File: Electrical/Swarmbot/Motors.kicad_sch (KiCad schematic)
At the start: 8 parts, among them J6 Motor 1, J7 Motor 2, U10 MPC17531A

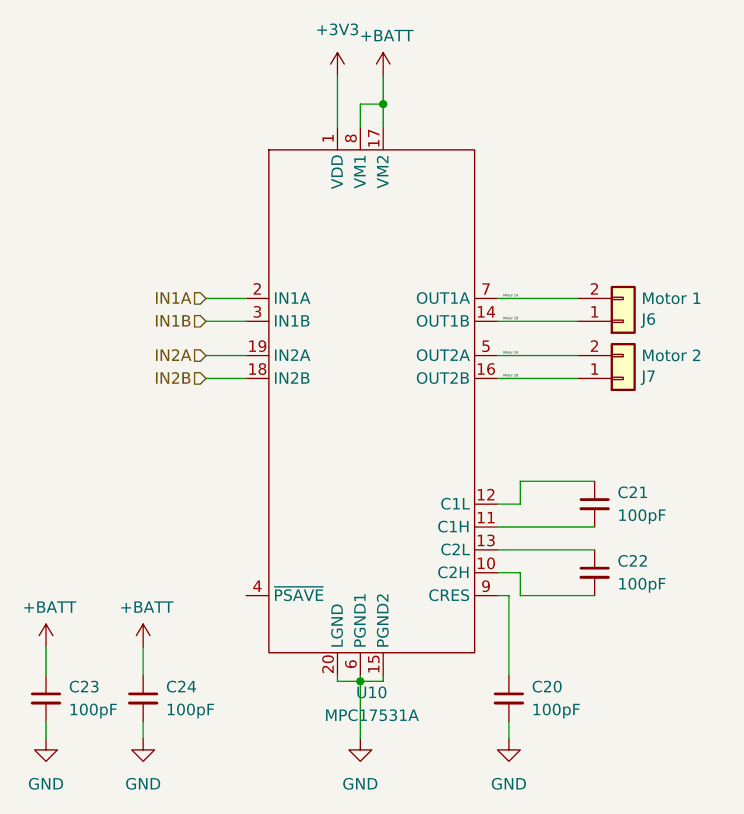
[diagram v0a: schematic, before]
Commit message: some little changes have been made
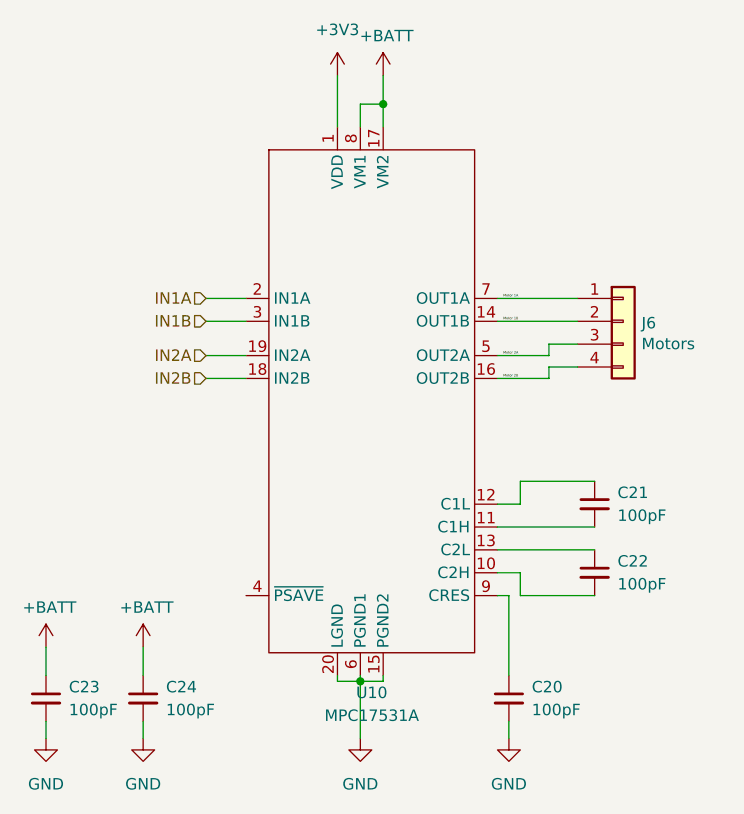
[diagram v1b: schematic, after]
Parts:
- removed J6: Motor 1, Connector_JST:JST_XH_B2B-XH-AM_1x02_P2.50mm_Vertical, symbol Connector_Generic:Conn_01x02
- removed J7: Motor 2, Connector_JST:JST_XH_B2B-XH-AM_1x02_P2.50mm_Vertical, symbol Connector_Generic:Conn_01x02
- added J6: Motors, Connector_JST:JST_XH_B4B-XH-AM_1x04_P2.50mm_Vertical, symbol Connector_Generic:Conn_01x04
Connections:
- net Motor 1A: now also J6.1 (Pin_1)
- net Motor 1B: now also J6.2 (Pin_2)
- net Motor 2A: now also J6.3 (Pin_3)
- net Motor 2B: now also J6.4 (Pin_4)
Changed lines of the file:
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@@
     (stroke (width 0) (type default) (color 0 0 0 0))
   )
-  (wire (pts (xy 126.365 83.185) (xy 135.255 83.185))
-    (stroke (width 0) (type default) (color 0 0 0 0))
-  )
-  (wire (pts (xy 126.365 85.725) (xy 135.255 85.725))
+  (wire (pts (xy 126.365 83.185) (xy 132.08 83.185))
+    (stroke (width 0) (type default) (color 0 0 0 0))
+  )
+  (wire (pts (xy 126.365 85.725) (xy 132.08 85.725))
     (stroke (width 0) (type default) (color 0 0 0 0))
   )
@@
   )
   (wire (pts (xy 128.905 109.855) (xy 137.16 109.855))
+    (stroke (width 0) (type default) (color 0 0 0 0))
+  )
+  (wire (pts (xy 132.08 81.915) (xy 132.08 83.185))
+    (stroke (width 0) (type default) (color 0 0 0 0))
+  )
+  (wire (pts (xy 132.08 84.455) (xy 132.08 85.725))
+    (stroke (width 0) (type default) (color 0 0 0 0))
+  )
+  (wire (pts (xy 135.255 81.915) (xy 132.08 81.915))
+    (stroke (width 0) (type default) (color 0 0 0 0))
+  )
+  (wire (pts (xy 135.255 84.455) (xy 132.08 84.455))
     (stroke (width 0) (type default) (color 0 0 0 0))
   )
@@
     (pin "2")
   )
-  (symbol (lib_id "Connector_Generic:Conn_01x02") (at 140.335 79.375 0) (mirror x) (unit 1)
-    (in_bom yes) (on_board yes)
-    (property "Reference" "J6" (id 0) (at 142.367 79.1718 0)
-      (effects (font (size 1.27 1.27)) (justify left))
-    )
-    (property "Value" "Motor 1" (id 1) (at 142.367 76.8604 0)
-      (effects (font (size 1.27 1.27)) (justify left))
-    )
-    (property "Footprint" "Connector_JST:JST_XH_B2B-XH-AM_1x02_P2.50mm_Vertical" (id 2) (at 140.335 79.375 0)
+  (symbol (lib_id "Connector_Generic:Conn_01x04") (at 140.335 79.375 0) (unit 1)
+    (in_bom yes) (on_board yes)
+    (property "Reference" "J6" (id 0) (at 142.367 79.5782 0)
+      (effects (font (size 1.27 1.27)) (justify left))
+    )
+    (property "Value" "Motors" (id 1) (at 142.367 81.8896 0)
+      (effects (font (size 1.27 1.27)) (justify left))
+    )
+    (property "Footprint" "Connector_JST:JST_XH_B4B-XH-AM_1x04_P2.50mm_Vertical" (id 2) (at 140.335 79.375 0)
       (effects (font (size 1.27 1.27)) hide)
     )
@@
     (pin "1")
     (pin "2")
-  )
-  (symbol (lib_id "Connector_Generic:Conn_01x02") (at 140.335 85.725 0) (mirror x) (unit 1)
-    (in_bom yes) (on_board yes)
-    (property "Reference" "J7" (id 0) (at 142.367 85.5218 0)
-      (effects (font (size 1.27 1.27)) (justify left))
-    )
-    (property "Value" "Motor 2" (id 1) (at 142.367 83.2104 0)
-      (effects (font (size 1.27 1.27)) (justify left))
-    )
-    (property "Footprint" "Connector_JST:JST_XH_B2B-XH-AM_1x02_P2.50mm_Vertical" (id 2) (at 140.335 85.725 0)
-      (effects (font (size 1.27 1.27)) hide)
-    )
-    (property "Datasheet" "~" (id 3) (at 140.335 85.725 0)
-      (effects (font (size 1.27 1.27)) hide)
-    )
-    (pin "1")
-    (pin "2")
+    (pin "3")
+    (pin "4")
   )
   (symbol (lib_id "MPC17531ATEJ - H Bridge:MPC17531A") (at 111.125 90.805 0) (unit 1)
